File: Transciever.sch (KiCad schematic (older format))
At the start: 0 parts

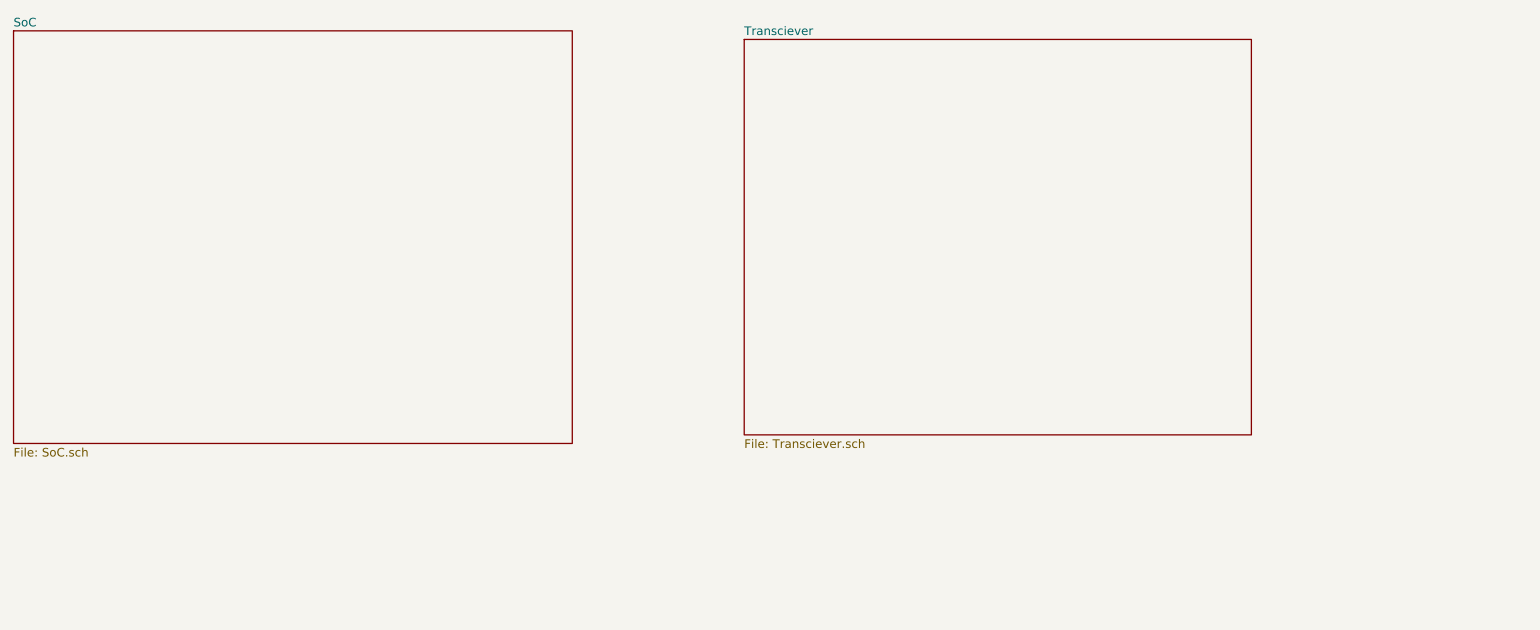
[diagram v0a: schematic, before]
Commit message: crot
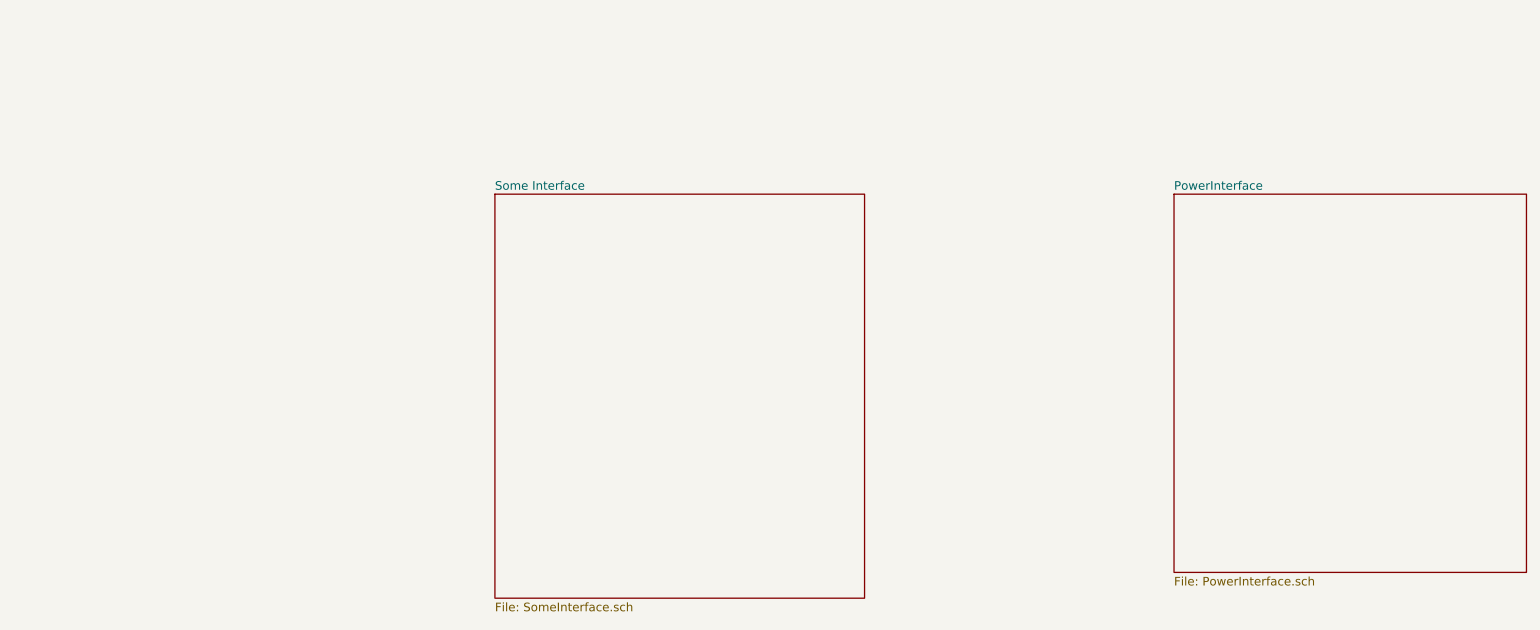
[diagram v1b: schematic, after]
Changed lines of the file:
@@
 $Descr A3 16535 11693
 encoding utf-8
-Sheet 1 11
+Sheet 9 11
 Title ""
 Date ""
@@
 $EndDescr
 $Sheet
-S 1650 1200 3250 2400
-U 5DE35227
-F0 "SoC" 50
-F1 "SoC.sch" 50
+S 4450 2150 2150 2350
+U 5DDB81DD
+F0 "Some Interface" 50
+F1 "SomeInterface.sch" 50
 $EndSheet
 $Sheet
-S 5900 1250 2950 2300
-U 5DDAC124
-F0 "Transciever" 50
-F1 "Transciever.sch" 50
+S 8400 2150 2050 2200
+U 5DDB8272
+F0 "PowerInterface" 50
+F1 "PowerInterface.sch" 50
 $EndSheet
 $EndSCHEMATC
